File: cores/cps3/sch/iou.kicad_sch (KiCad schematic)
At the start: 1 part

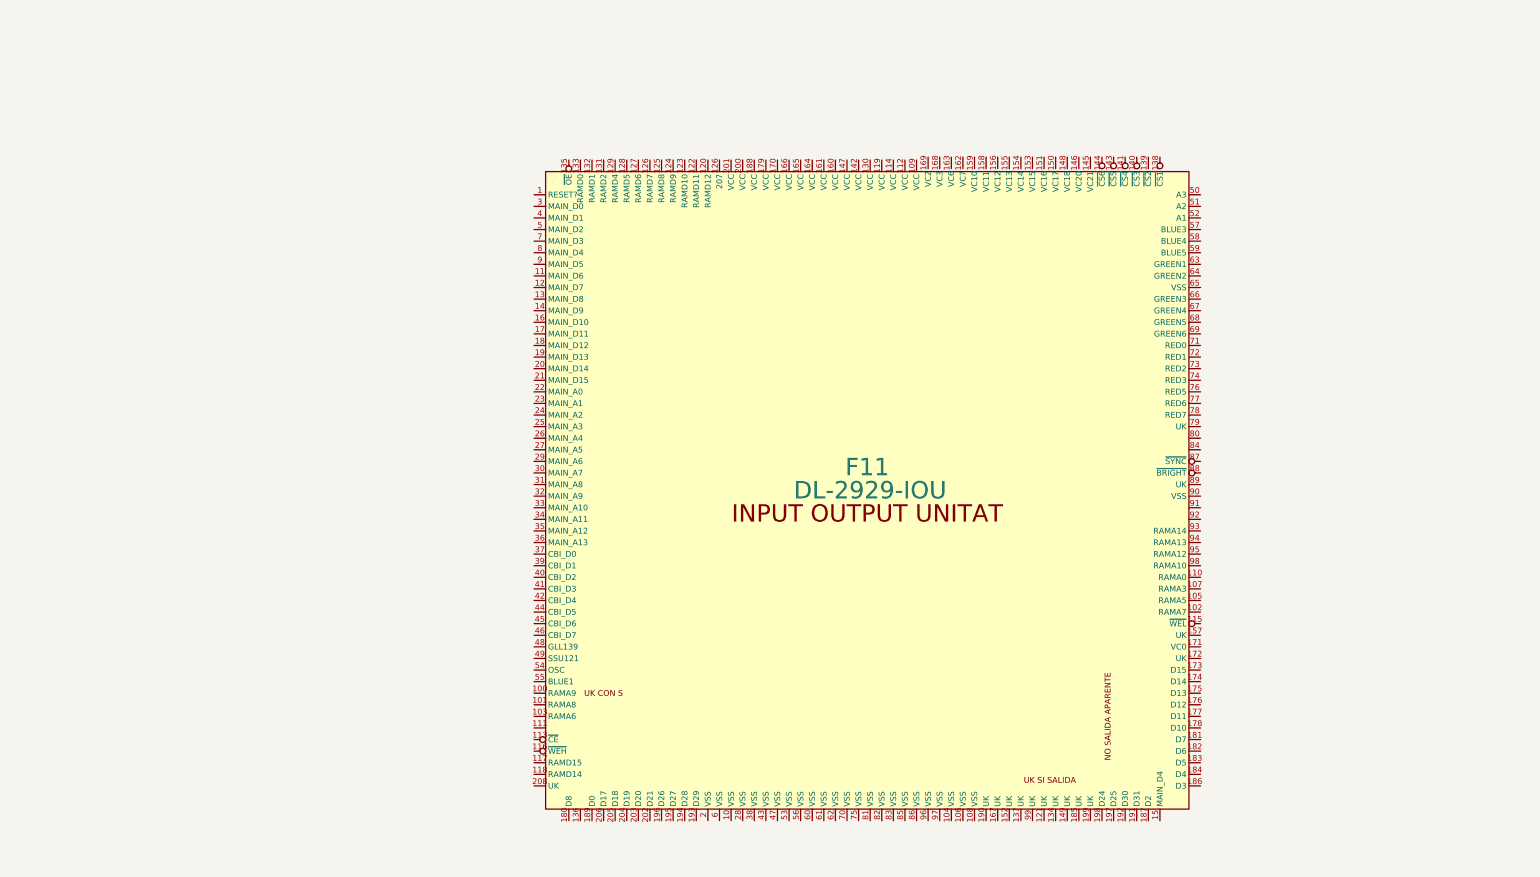
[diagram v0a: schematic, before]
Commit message: uptate_ns
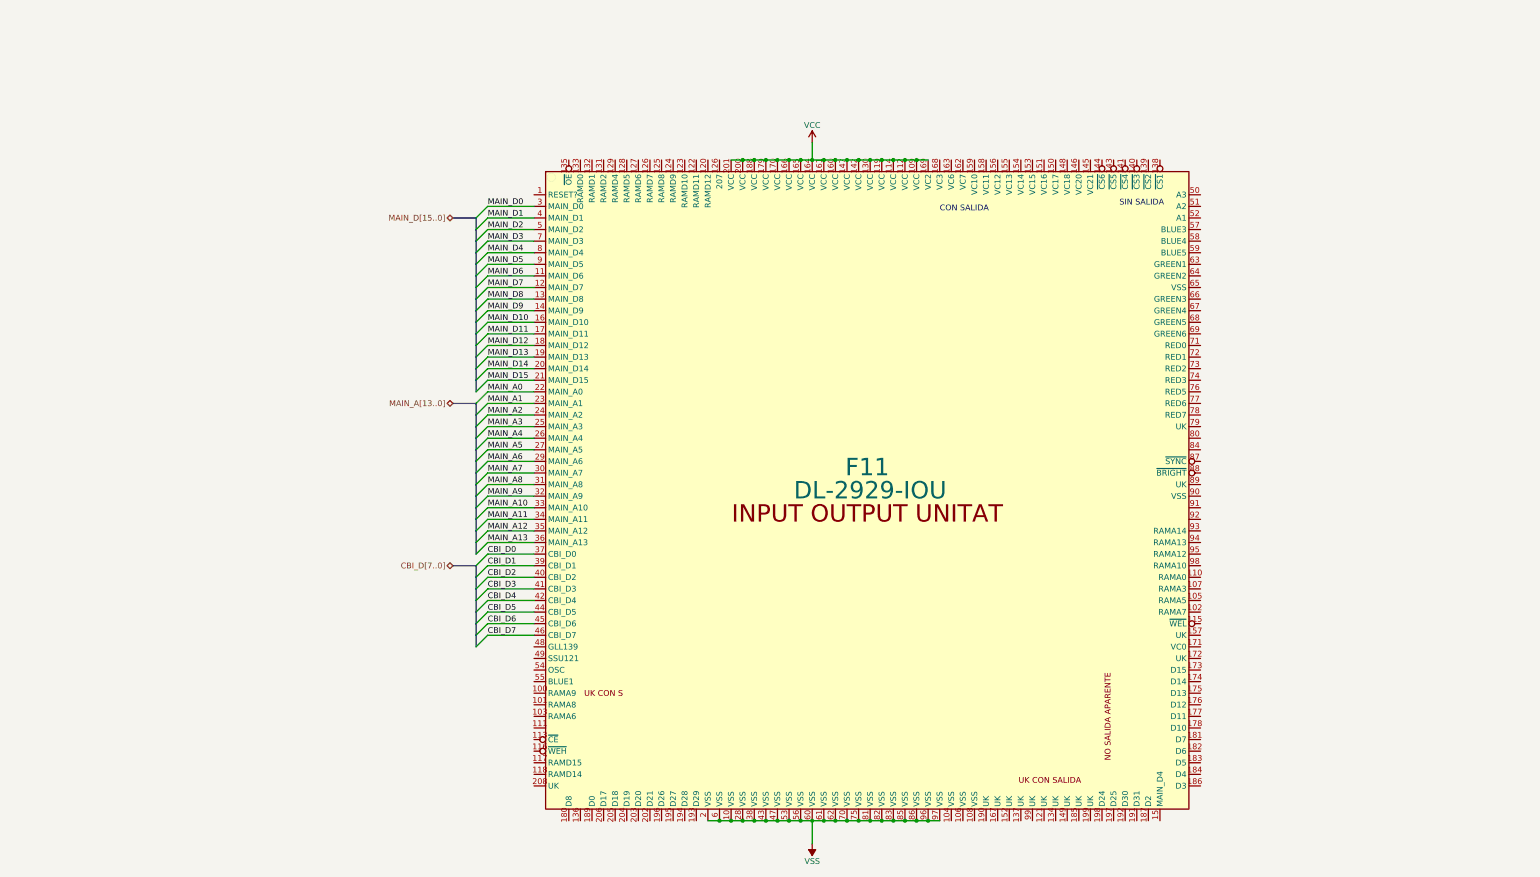
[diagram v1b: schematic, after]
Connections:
- net VSS: now reaches F11.10 (VSS)
- net VSS: now also F11.2 (VSS), F11.28 (VSS), F11.38 (VSS), F11.43 (VSS), F11.47 (VSS), F11.53 (VSS), F11.56 (VSS), F11.6 (VSS), F11.60 (VSS), F11.61 (VSS), F11.62 (VSS), F11.70 (VSS), F11.75 (VSS), F11.81 (VSS), F11.82 (VSS), F11.83 (VSS), F11.85 (VSS), F11.86 (VSS), F11.96 (VSS), F11.97 (VSS)
- net VCC: now reaches F11.109 (VCC)
- net VCC: now also F11.112 (VCC), F11.114 (VCC), F11.119 (VCC), F11.130 (VCC), F11.142 (VCC), F11.147 (VCC), F11.160 (VCC), F11.161 (VCC), F11.164 (VCC), F11.165 (VCC), F11.166 (VCC), F11.169 (VC2), F11.170 (VCC), F11.179 (VCC), F11.188 (VCC), F11.200 (VCC), F11.201 (VCC)
- net MAIN_D6: now reaches F11.11 (MAIN_D6)
- net MAIN_D7: now reaches F11.12 (MAIN_D7)
- net MAIN_D8: now reaches F11.13 (MAIN_D8)
- net MAIN_D9: now reaches F11.14 (MAIN_D9)
- net MAIN_D10: now reaches F11.16 (MAIN_D10)
- net MAIN_D11: now reaches F11.17 (MAIN_D11)
- net MAIN_D12: now reaches F11.18 (MAIN_D12)
- net MAIN_D13: now reaches F11.19 (MAIN_D13)
- net MAIN_D14: now reaches F11.20 (MAIN_D14)
- net MAIN_D15: now reaches F11.21 (MAIN_D15)
- net MAIN_A0: now reaches F11.22 (MAIN_A0)
- net MAIN_A1: now reaches F11.23 (MAIN_A1)
- net MAIN_A2: now reaches F11.24 (MAIN_A2)
- net MAIN_A3: now reaches F11.25 (MAIN_A3)
- net MAIN_A4: now reaches F11.26 (MAIN_A4)
- net MAIN_A5: now reaches F11.27 (MAIN_A5)
- net MAIN_A6: now reaches F11.29 (MAIN_A6)
- net MAIN_D0: now reaches F11.3 (MAIN_D0)
- net MAIN_A7: now reaches F11.30 (MAIN_A7)
- net MAIN_A8: now reaches F11.31 (MAIN_A8)
- net MAIN_A9: now reaches F11.32 (MAIN_A9)
- net MAIN_A10: now reaches F11.33 (MAIN_A10)
- net MAIN_A11: now reaches F11.34 (MAIN_A11)
- net MAIN_A12: now reaches F11.35 (MAIN_A12)
- net MAIN_A13: now reaches F11.36 (MAIN_A13)
- net CBI_D0: now reaches F11.37 (CBI_D0)
- net CBI_D1: now reaches F11.39 (CBI_D1)
- net MAIN_D1: now reaches F11.4 (MAIN_D1)
- net CBI_D2: now reaches F11.40 (CBI_D2)
- net CBI_D3: now reaches F11.41 (CBI_D3)
- net CBI_D4: now reaches F11.42 (CBI_D4)
- net CBI_D5: now reaches F11.44 (CBI_D5)
- net CBI_D6: now reaches F11.45 (CBI_D6)
- net CBI_D7: now reaches F11.46 (CBI_D7)
- net MAIN_D2: now reaches F11.5 (MAIN_D2)
- net MAIN_D3: now reaches F11.7 (MAIN_D3)
- net MAIN_D4: now reaches F11.8 (MAIN_D4)
- net MAIN_D5: now reaches F11.9 (MAIN_D5)
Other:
- note added: "CON SALIDA"
- note added: "SIN SALIDA"

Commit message: update_cps3
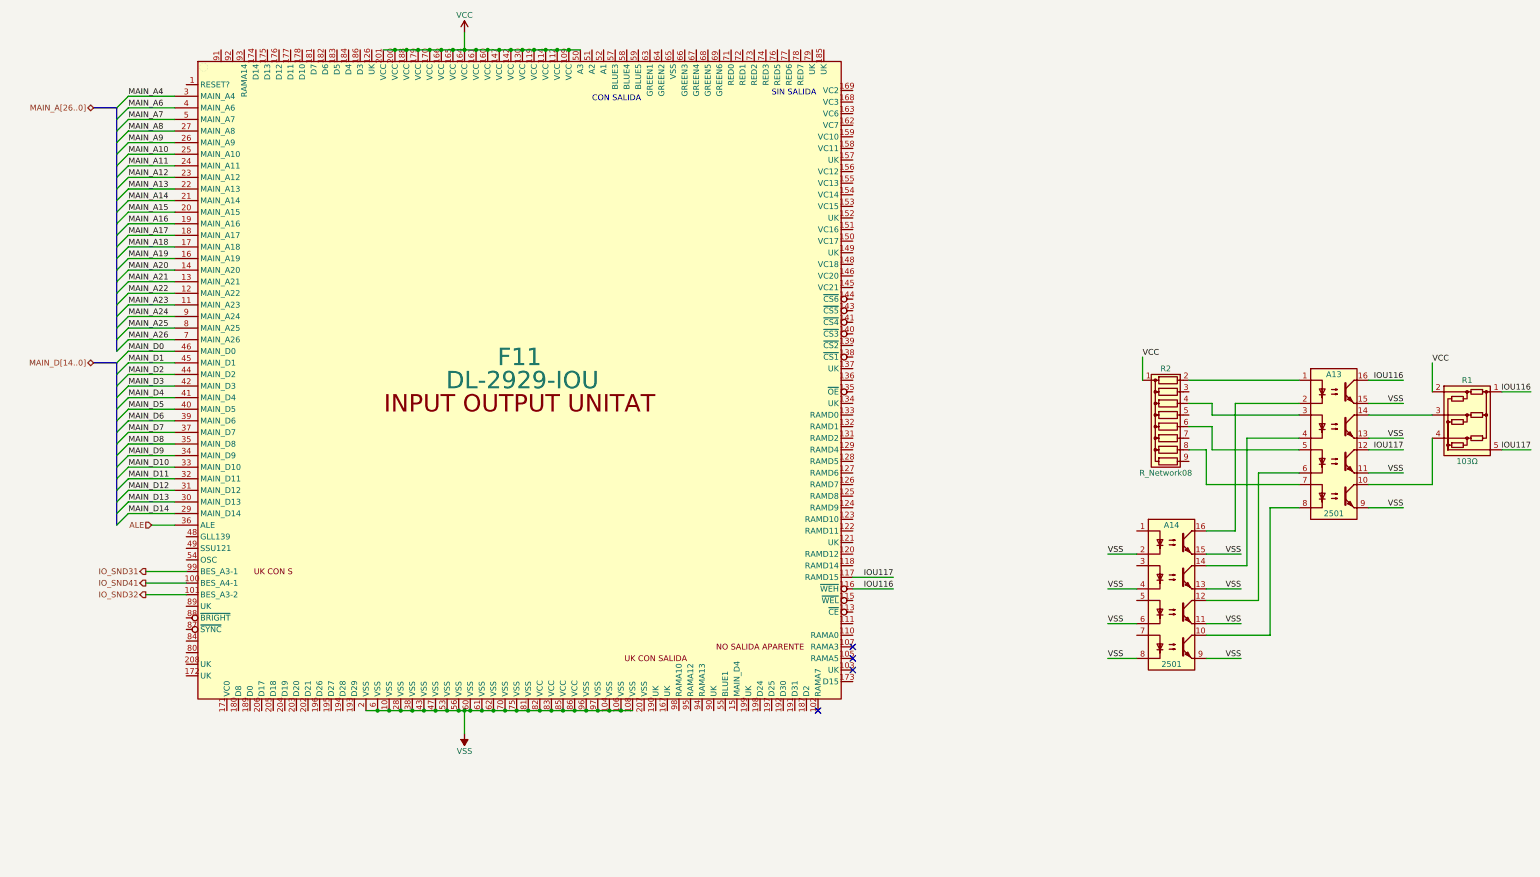
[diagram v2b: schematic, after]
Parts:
- added A13, A14: 2501, symbol Nec:2501
- added R1: 103Ω, Resistor_THT:R_Array_SIP5, symbol Device:R_Network_Dividers_x03_SIP
- added R2: R_Network08, Resistor_THT:R_Array_SIP9, symbol Device:R_Network08
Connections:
- net CBI_D0 is gone; now on net MAIN_D7: F11.37 (MAIN_D7)
- net CBI_D1 is gone; now on net MAIN_D6: F11.39 (MAIN_D6)
- net CBI_D2 is gone; now on net MAIN_D5: F11.40 (MAIN_D5)
- net CBI_D3 is gone; now on net MAIN_D4: F11.41 (MAIN_D4)
- net CBI_D4 is gone; now on net MAIN_D3: F11.42 (MAIN_D3)
- net CBI_D5 is gone; now on net MAIN_D2: F11.44 (MAIN_D2)
- net CBI_D6 is gone; now on net MAIN_D1: F11.45 (MAIN_D1)
- net CBI_D7 is gone; now on net MAIN_D0: F11.46 (MAIN_D0)
- net MAIN_A0 is gone; now on net MAIN_A13: F11.22 (MAIN_A13)
- net MAIN_A1 is gone; now on net MAIN_A12: F11.23 (MAIN_A12)
- net MAIN_A2 is gone; now on net MAIN_A11: F11.24 (MAIN_A11)
- net MAIN_A3 is gone; now on net MAIN_A10: F11.25 (MAIN_A10)
- net MAIN_A5 is gone; now on net MAIN_A8: F11.27 (MAIN_A8)
- net MAIN_A10: no longer F11.33 (MAIN_A10)
- net MAIN_A11: no longer F11.34 (MAIN_A11)
- net MAIN_A12: no longer F11.35 (MAIN_A12)
- net MAIN_A13: no longer F11.36 (MAIN_A13)
- net MAIN_A4: now also F11.3 (MAIN_A4); no longer F11.26 (MAIN_A4)
- net MAIN_A6: now also F11.4 (MAIN_A6); no longer F11.29 (MAIN_A6)
- net MAIN_A7: now also F11.5 (MAIN_A7); no longer F11.30 (MAIN_A7)
- net MAIN_A8: no longer F11.31 (MAIN_A8)
- net MAIN_A9: now also F11.26 (MAIN_A9); no longer F11.32 (MAIN_A9)
- net MAIN_D0: no longer F11.3 (MAIN_D0)
- net MAIN_D1: no longer F11.4 (MAIN_D1)
- net MAIN_D10: now also F11.33 (MAIN_D10); no longer F11.16 (MAIN_D10)
- net MAIN_D11: now also F11.32 (MAIN_D11); no longer F11.17 (MAIN_D11)
- net MAIN_D12: now also F11.31 (MAIN_D12); no longer F11.18 (MAIN_D12)
- net MAIN_D13: now also F11.30 (MAIN_D13); no longer F11.19 (MAIN_D13)
- net MAIN_D14: now also F11.29 (MAIN_D14); no longer F11.20 (MAIN_D14)
- net MAIN_D2: no longer F11.5 (MAIN_D2)
- net MAIN_D3: no longer F11.7 (MAIN_D3)
- net MAIN_D4: no longer F11.8 (MAIN_D4)
- net MAIN_D5: no longer F11.9 (MAIN_D5)
- net MAIN_D6: no longer F11.11 (MAIN_D6)
- net MAIN_D7: no longer F11.12 (MAIN_D7)
- net MAIN_D8: now also F11.35 (MAIN_D8); no longer F11.13 (MAIN_D8)
- net MAIN_D9: now also F11.34 (MAIN_D9); no longer F11.14 (MAIN_D9)
- net VCC: now also F11.50 (A3), R1.2 (R1), R2.1 (common); no longer F11.169 (VC2)
- net VSS: now also F11.104 (VSS), F11.106 (VSS), F11.108 (VSS), A13.11, A13.13, A13.15, A13.9, A14.11, A14.13, A14.15, A14.2, A14.4, A14.6, A14.8, A14.9
- net IO_SND41: now reaches F11.100 (BES_A4-1)
- net IO_SND32: now reaches F11.101 (BES_A3-2)
- net IOU116: now reaches F11.116 (~{WEH})
- net IOU116: now also A13.16, R1.1 (COM1)
- net IOU117: now reaches F11.117 (RAMD15)
- net IOU117: now also A13.12, R1.5 (COM2)
- net IO_SND31: now reaches F11.99 (BES_A3-1)
- net MAIN_D15 renamed MAIN_A14
- new net: A13.1, R2.2 (R1)
- new net: A13.10, R1.4 (R3)
- new net: A13.14, R1.3 (R2)
- new net: A13.2, A14.16
- new net: A13.3, R2.4 (R3)
- new net: A13.4, A14.14
- new net: A13.5, R2.6 (R5)
- new net: A13.6, A14.12
- new net: A13.7, R2.8 (R7)
- new net: A13.8, A14.10
- new net ALE: F11.36 (ALE)
- new net MAIN_A15: F11.20 (MAIN_A15)
- new net MAIN_A16: F11.19 (MAIN_A16)
- new net MAIN_A17: F11.18 (MAIN_A17)
- new net MAIN_A18: F11.17 (MAIN_A18)
- new net MAIN_A19: F11.16 (MAIN_A19)
- new net MAIN_A20: F11.14 (MAIN_A20)
- new net MAIN_A21: F11.13 (MAIN_A21)
- new net MAIN_A22: F11.12 (MAIN_A22)
- new net MAIN_A23: F11.11 (MAIN_A23)
- new net MAIN_A24: F11.9 (MAIN_A24)
- new net MAIN_A25: F11.8 (MAIN_A25)
- new net MAIN_A26: F11.7 (MAIN_A26)
- no-connect marks 0 -> 4
